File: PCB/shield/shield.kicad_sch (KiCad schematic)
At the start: 19 parts, among them J1 QTR-8A, J10 ESP32_left_m, J11 ESP32_right_m, J13 Conn_01x06, J14 Domino, J15 Domino, J2 QMC5883L, J3 Servo, J4 Domino, J5 Joystick, J6 OLED, J8 ESP32_left_f, J9 ESP32_right_f, U1 YAAJ_DCDC_StepDown_LM2596

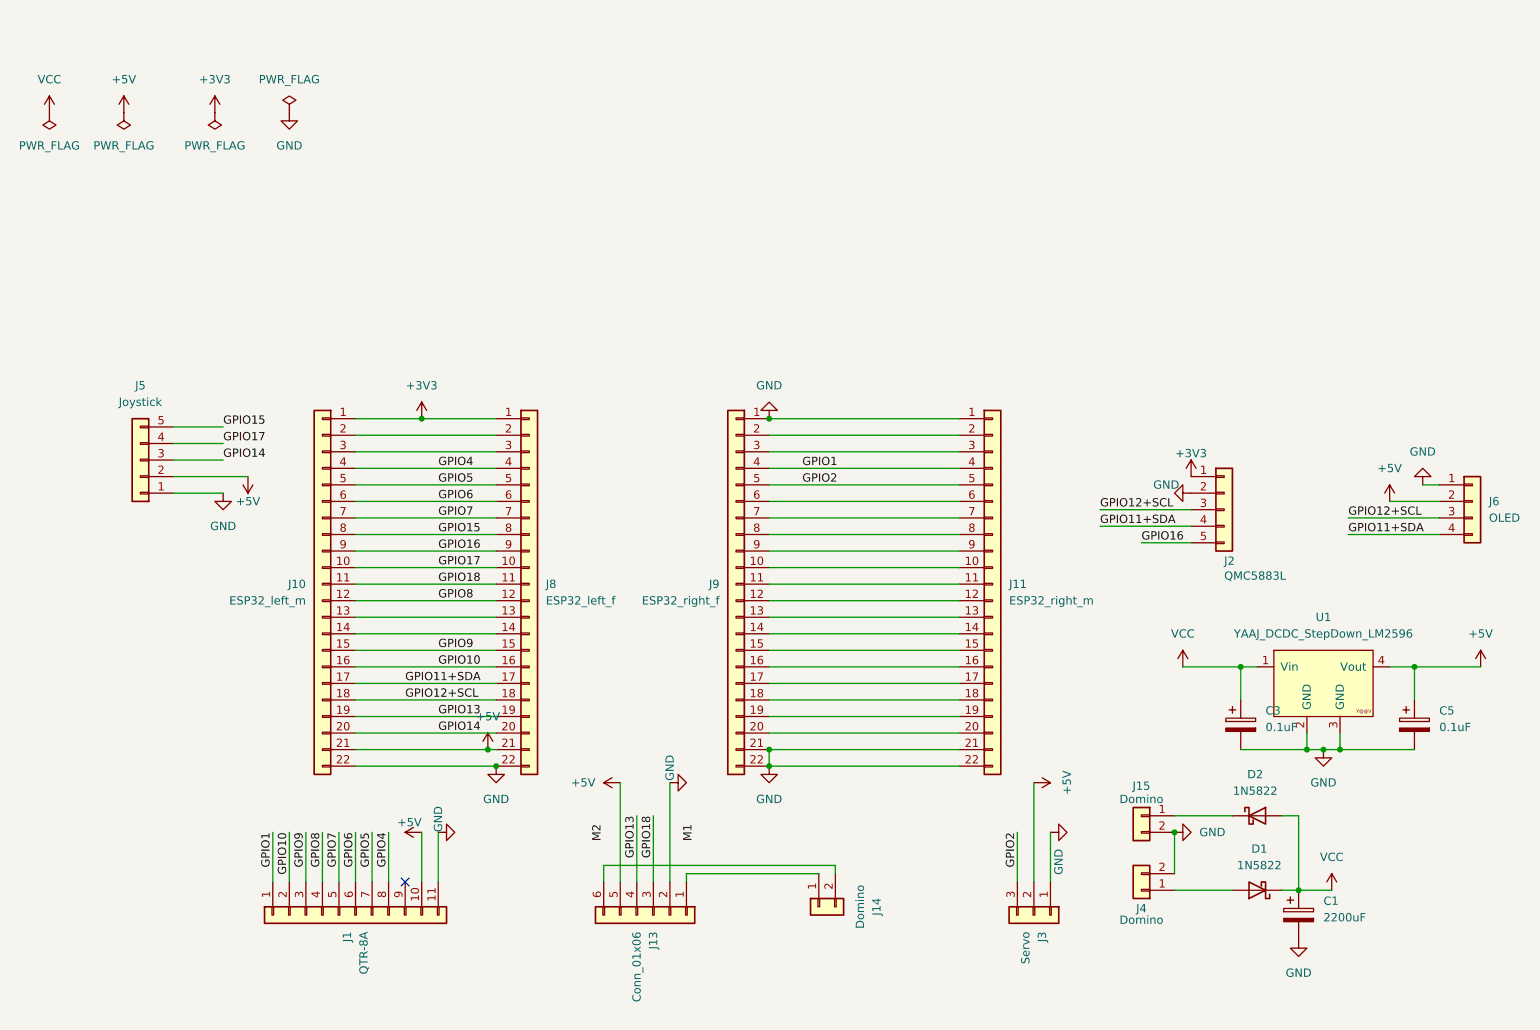
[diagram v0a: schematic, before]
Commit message: wip: commit to change workplace
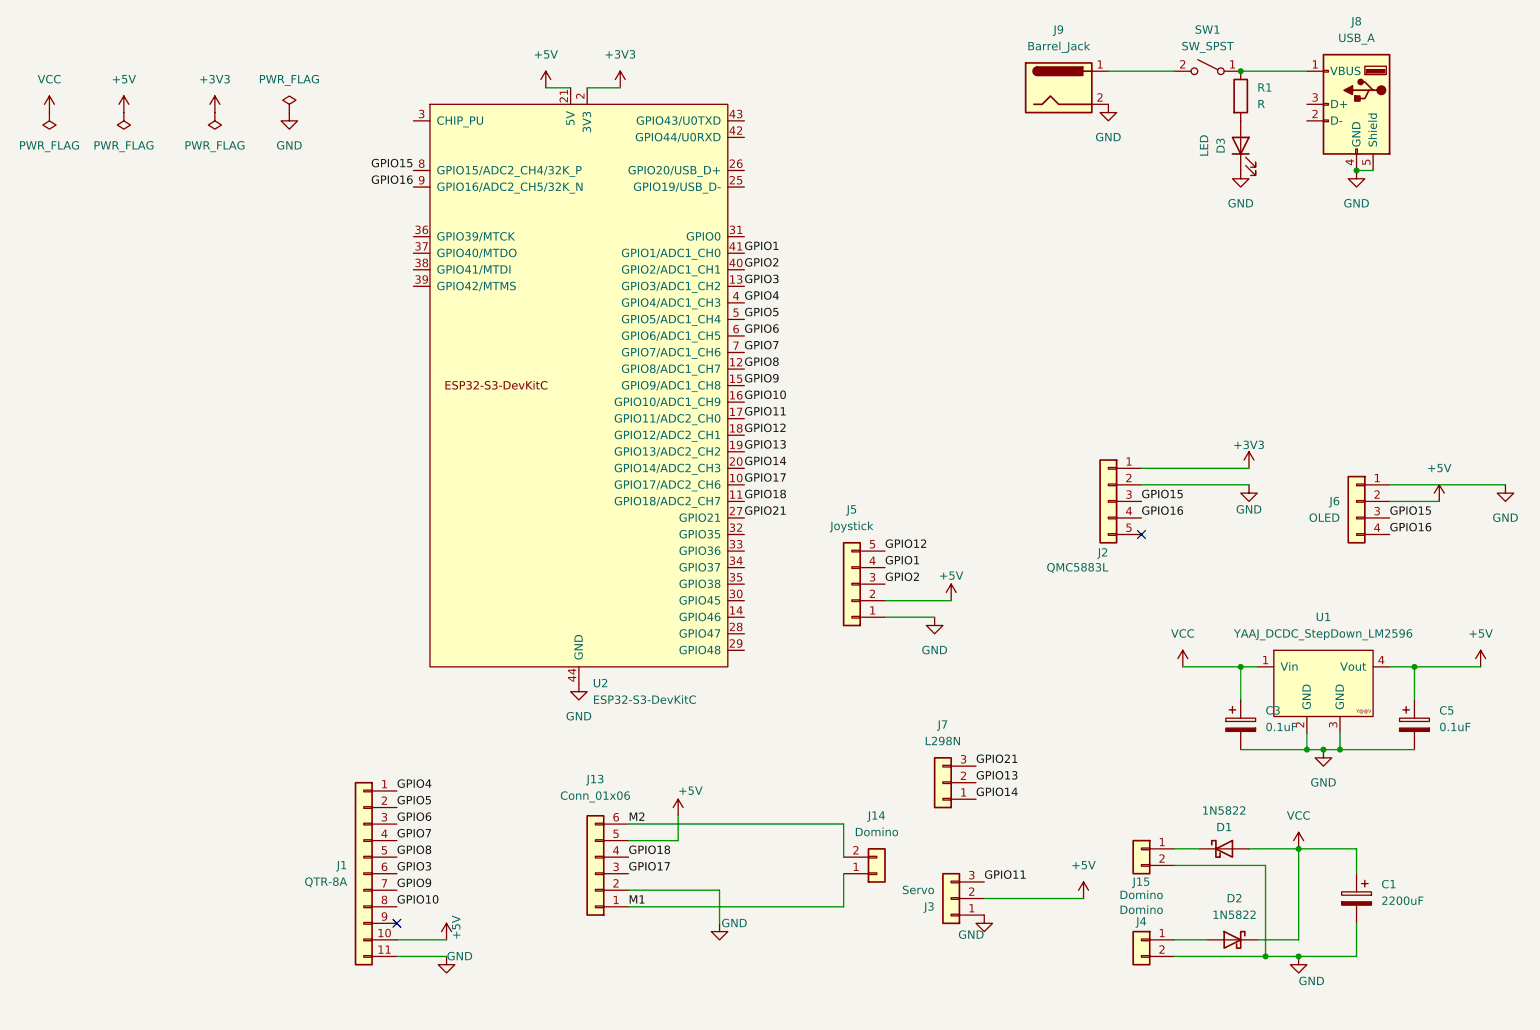
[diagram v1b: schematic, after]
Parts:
- removed J10: ESP32_left_m, Connector_PinHeader_2.54mm:PinHeader_1x22_P2.54mm_Vertical, symbol Connector_Generic:Conn_01x22
- removed J11: ESP32_right_m, Connector_PinHeader_2.54mm:PinHeader_1x22_P2.54mm_Vertical, symbol Connector_Generic:Conn_01x22
- removed J8: ESP32_left_f, Connector_PinSocket_2.54mm:PinSocket_1x22_P2.54mm_Vertical, symbol Connector_Generic:Conn_01x22
- removed J9: ESP32_right_f, Connector_PinSocket_2.54mm:PinSocket_1x22_P2.54mm_Vertical, symbol Connector_Generic:Conn_01x22
- added D3: LED, symbol Device:LED
- added J7: L298N, Connector_JST:JST_XH_B3B-XH-A_1x03_P2.50mm_Vertical, symbol Connector_Generic:Conn_01x03
- added J8: USB_A, symbol Connector:USB_A
- added J9: Barrel_Jack, symbol Connector:Barrel_Jack
- added R1: R, symbol Device:R
- added SW1: SW_SPST, symbol Switch:SW_SPST
- added U2: ESP32-S3-DevKitC, PCM_Espressif:ESP32-S3-DevKitC, symbol PCM_Espressif:ESP32-S3-DevKitC
- C3, C5: footprint Capacitor_SMD:C_0805_2012Metric_Pad1.18x1.45mm_HandSolder -> Capacitor_THT:CP_Radial_D5.0mm_P2.50mm
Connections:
- net GPIO11+SDA is gone; now on net GPIO16: J2.4 (Pin_4), J6.4 (Pin_4)
- net GPIO12+SCL is gone; now on net GPIO15: J2.3 (Pin_3), J6.3 (Pin_3)
- net +3V3: now also U2.1 (3V3), U2.2 (3V3)
- net +5V: now also U2.21 (5V)
- net GND: now also D3.1 (K), J8.4 (GND), J8.5 (Shield), J9.2, U2.22 (GND), U2.23 (GND), U2.24 (GND), U2.44 (GND)
- net GPIO1: now also J5.4 (Pin_4), U2.41 (GPIO1/ADC1_CH0); no longer J1.1 (Pin_1)
- net GPIO10: now also J1.8 (Pin_8), U2.16 (GPIO10/ADC1_CH9); no longer J1.2 (Pin_2)
- net GPIO13: now also J7.2 (Pin_2), U2.19 (GPIO13/ADC2_CH2); no longer J13.4 (Pin_4)
- net GPIO14: now also J7.1 (Pin_1), U2.20 (GPIO14/ADC2_CH3); no longer J5.3 (Pin_3)
- net GPIO15: now also U2.8 (GPIO15/ADC2_CH4/32K_P); no longer J5.5 (Pin_5)
- net GPIO16: now also U2.9 (GPIO16/ADC2_CH5/32K_N); no longer J2.5 (Pin_5)
- net GPIO17: now also J13.3 (Pin_3), U2.10 (GPIO17/ADC2_CH6); no longer J5.4 (Pin_4)
- net GPIO18: now also J13.4 (Pin_4), U2.11 (GPIO18/ADC2_CH7); no longer J13.3 (Pin_3)
- net GPIO2: now also J5.3 (Pin_3), U2.40 (GPIO2/ADC1_CH1); no longer J3.3 (Pin_3)
- net GPIO4: now also J1.1 (Pin_1), U2.4 (GPIO4/ADC1_CH3); no longer J1.8 (Pin_8)
- net GPIO5: now also J1.2 (Pin_2), U2.5 (GPIO5/ADC1_CH4); no longer J1.7 (Pin_7)
- net GPIO6: now also J1.3 (Pin_3), U2.6 (GPIO6/ADC1_CH5); no longer J1.6 (Pin_6)
- net GPIO7: now also J1.4 (Pin_4), U2.7 (GPIO7/ADC1_CH6); no longer J1.5 (Pin_5)
- net GPIO8: now also J1.5 (Pin_5), U2.12 (GPIO8/ADC1_CH7); no longer J1.4 (Pin_4)
- net GPIO9: now also J1.7 (Pin_7), U2.15 (GPIO9/ADC1_CH8); no longer J1.3 (Pin_3)
- net M1: now also J13.1 (Pin_1), J14.1 (Pin_1)
- net M2: now also J13.6 (Pin_6), J14.2 (Pin_2)
- net VCC: now also D1.2 (A), D2.1 (K); no longer D1.1 (K), D2.2 (A)
- net at J4.1 (Pin_1): now also D2.2 (A); no longer D1.2 (A)
- net at J15.1 (Pin_1): now also D1.1 (K); no longer D2.1 (K)
- new net: J8.1 (VBUS), R1.1, SW1.1 (A)
- new net: J9.1, SW1.2 (B)
- new net: D3.2 (A), R1.2
- new net GPIO11: J3.3 (Pin_3), U2.17 (GPIO11/ADC2_CH0)
- new net GPIO12: J5.5 (Pin_5), U2.18 (GPIO12/ADC2_CH1)
- new net GPIO21: J7.3 (Pin_3), U2.27 (GPIO21)
- new net GPIO3: J1.6 (Pin_6), U2.13 (GPIO3/ADC1_CH2)
- no-connect marks 1 -> 2
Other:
- moved on the sheet: C1, D1, D2, J1, J13, J14, J15, J2, J3, J4, J5, J6

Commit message: wip: commit to change workspace
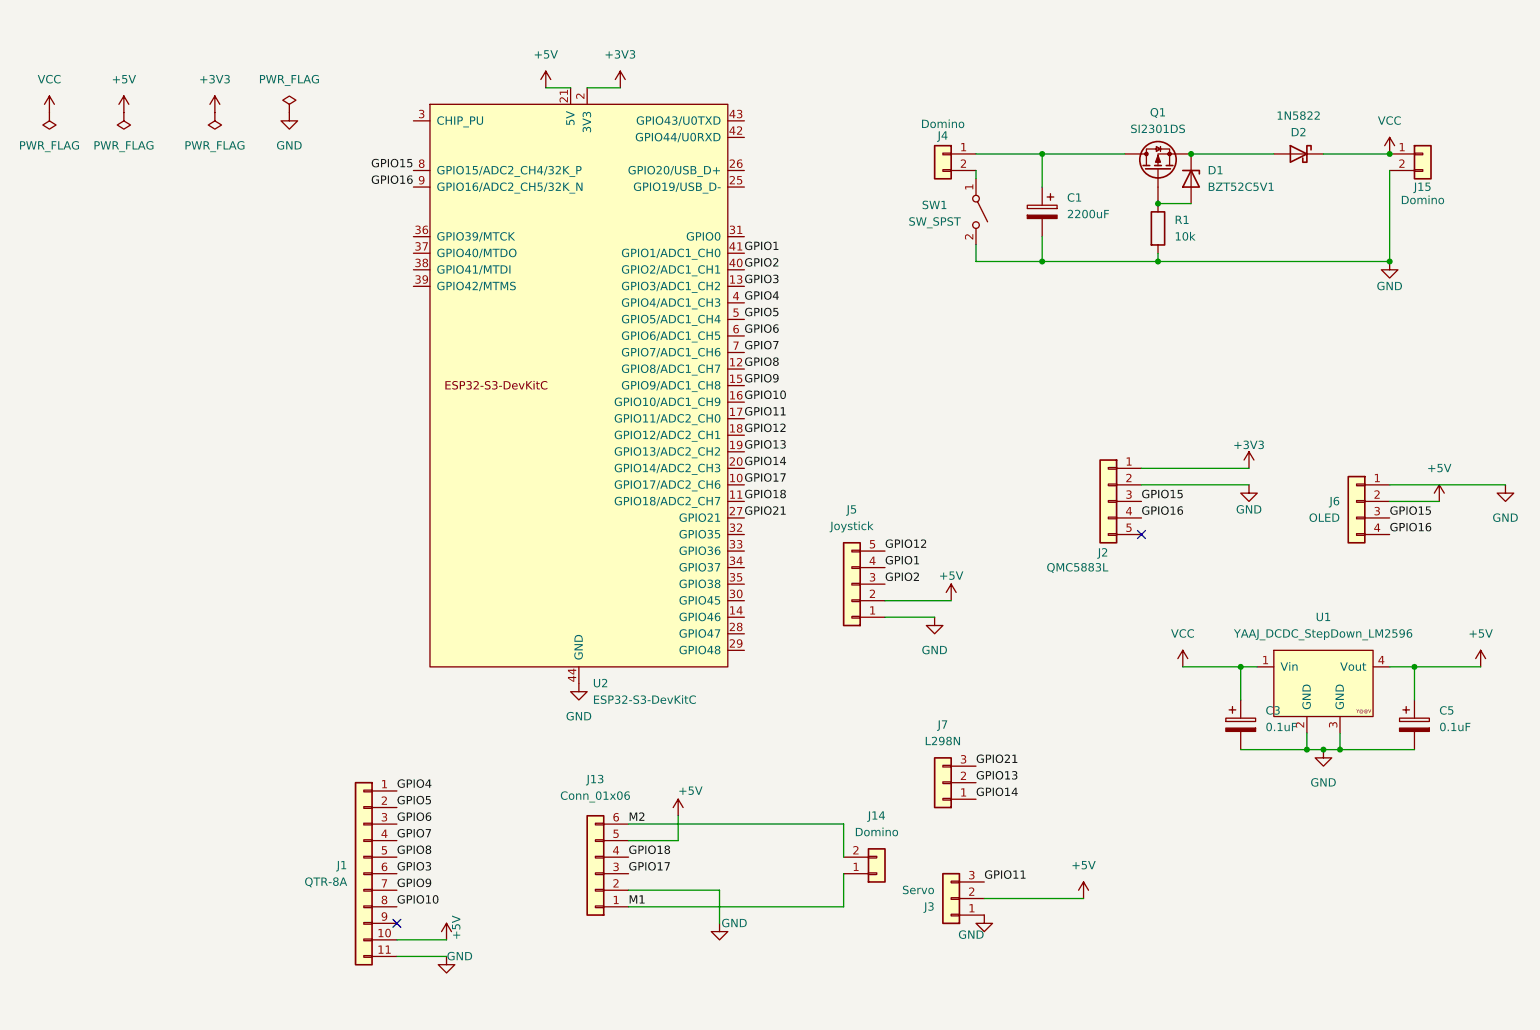
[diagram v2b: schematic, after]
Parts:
- removed D1: 1N5822, Diode_THT:D_DO-201AD_P15.24mm_Horizontal, symbol Diode:1N5822
- removed D3: LED, symbol Device:LED
- removed J8: USB_A, symbol Connector:USB_A
- removed J9: Barrel_Jack, symbol Connector:Barrel_Jack
- added D1: BZT52C5V1, Diode_SMD:D_SOD-123, symbol Device:D_Zener
- added Q1: SI2301DS, Package_TO_SOT_SMD:SOT-23-3, symbol Device:Q_PMOS
- R1: value R -> 10k; footprint (none) -> Resistor_SMD:R_0603_1608Metric_Pad0.98x0.95mm_HandSolder
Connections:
- net GND: now also R1.2, SW1.2 (B); no longer J4.2 (Pin_2)
- net VCC: now also J15.1 (Pin_1); no longer C1.1
- net at R1.1: now also D1.2 (A), Q1.G; no longer SW1.1 (A)
- net at D2.2 (A): now also D1.1 (K), Q1.S; no longer J4.1 (Pin_1)
- new net: C1.1, J4.1 (Pin_1), Q1.D
- new net: J4.2 (Pin_2), SW1.1 (A)
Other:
- moved on the sheet: C1, J15, J4
